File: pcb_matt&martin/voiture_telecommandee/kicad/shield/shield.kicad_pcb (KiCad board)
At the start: 2 copper layers, 100 x 100 mm, 13 parts, among them J2 Bluetooth, U1 COM-09032

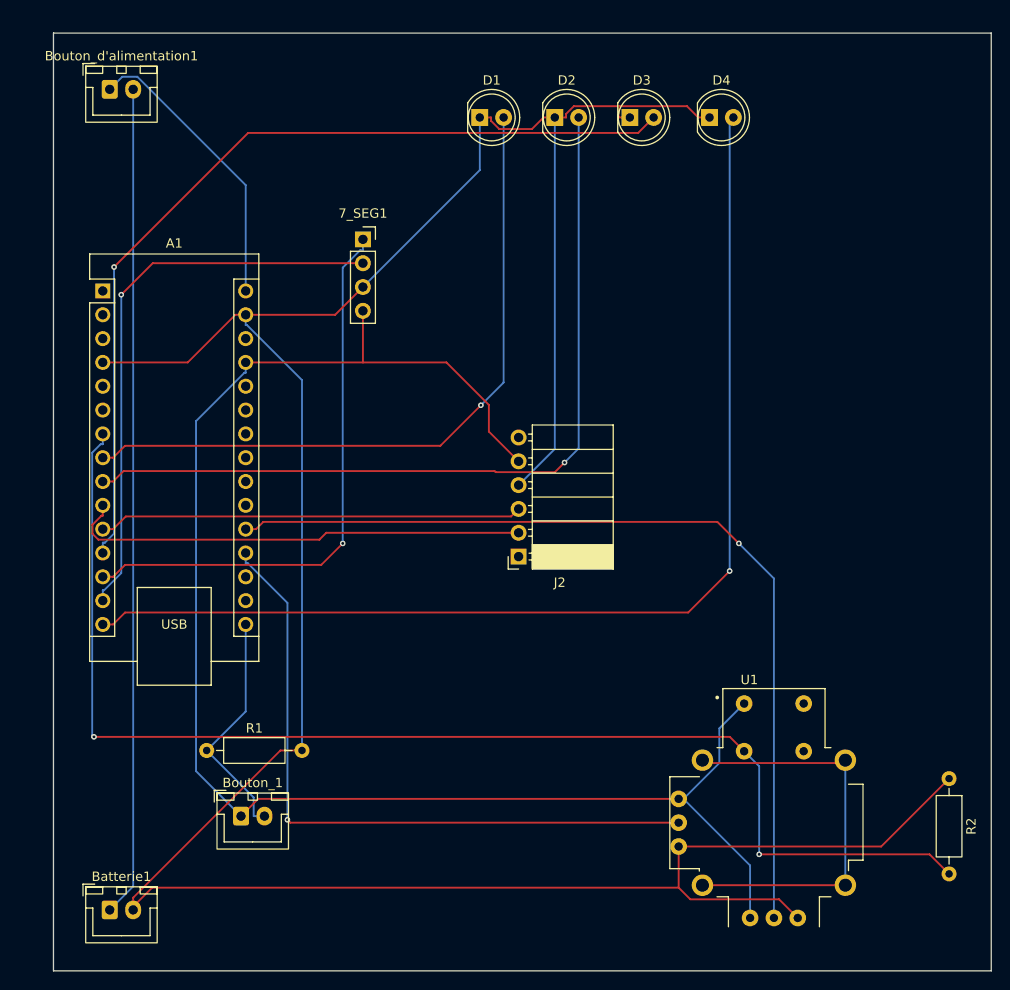
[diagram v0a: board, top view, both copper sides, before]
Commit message: bon euuuuu y'a bcp de changements
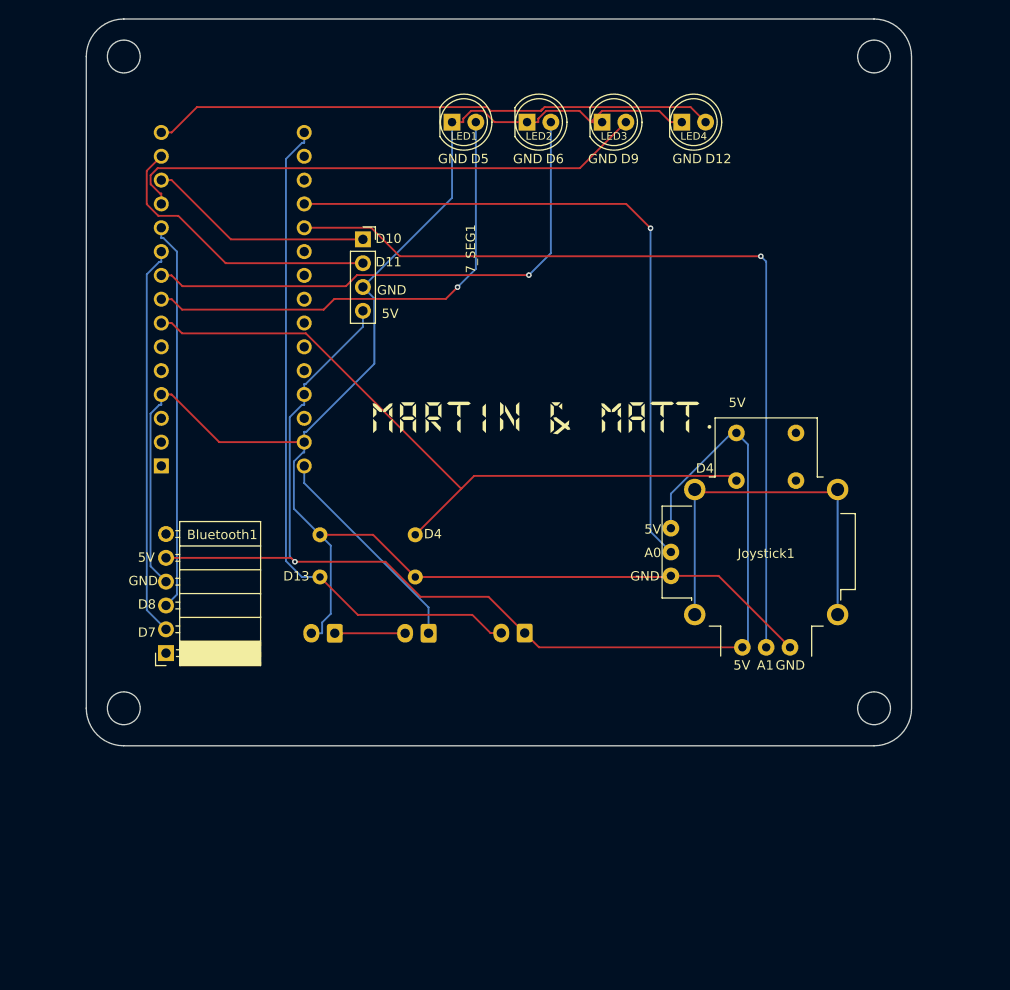
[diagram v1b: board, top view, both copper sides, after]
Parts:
- ARDUINO1: renamed from A1; moved to B.Cu
- Batterie1, R1, R2: moved to B.Cu
- Bouton1: renamed from Bouton_1; moved to B.Cu
- Btn_alim1: renamed from Bouton_d'alimentation1; moved to B.Cu
- moved R2 71.9 mm to (116.4, 104.0), turned to 0 degrees
- moved Btn_alim1 67.2 mm to (128.0, 114.5), turned to 180 degrees
- moved Bluetooth1 39.0 mm to (100.0, 116.6)
- moved Batterie1 38.0 mm to (118.0, 114.5), turned to 180 degrees
- moved Bouton1 36.0 mm to (138.2, 114.5), turned to 180 degrees
- moved Joystick1 28.9 mm to (164.0, 105.8)
- moved R1 22.1 mm to (116.4, 108.5)
- moved ARDUINO1 19.7 mm to (99.5, 96.7)
- moved LED1 3.00 mm to (130.5, 60.0)
- moved LED2 3.00 mm to (138.5, 60.0)
- moved LED3 3.00 mm to (146.5, 60.0)
- moved LED4 3.00 mm to (155.0, 60.0)
- renumbered J2 to Bluetooth1, U1 to Joystick1, D1 to LED1, D2 to LED2, D3 to LED3, D4 to LED4
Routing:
- net GND: track 308.6 -> 188.8 mm
- net /BTN_BATT_IN: track 88.5 -> 7.50 mm
- net /<NO NET>: track 136.5 -> 76.4 mm, vias 2 -> 0
- net /LED_4: track 117.7 -> 60.4 mm, vias 1 -> 0
- net /BTN_1: track 25.4 -> 72.8 mm
- net /LED_3: track 95.3 -> 56.6 mm, vias 1 -> 0
- net +5V: track 169.7 -> 132.8 mm, vias 0 -> 1
- net /7_SEG_CLK: track 60.5 -> 24.1 mm, vias 1 -> 0
- net /LED_2: track 87.9 -> 57.4 mm
- net /7_SEG_DIO: track 60.7 -> 31.4 mm, vias 1 -> 0
- net /LED_1: track 74.3 -> 51.4 mm
- net /BTN_BATT_OUT: track 31.1 -> 23.3 mm
- net /BTH_RX: track 49.6 -> 41.9 mm
- net /BTH_TX: track 45.2 -> 41.6 mm
- net /H2: track 95.3 -> 91.9 mm
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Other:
- board size 100 x 100 mm -> 88 x 77.5 mm
- board text added: "5V"
- board text added: "<->"
- board text added: "A0"
- board text added: "A1"
- board text added: "D10"
- board text added: "D11"
- board text added: "D12"
- board text added: "D13"
- board text added: "D4"
- board text added: "D5"
- board text added: "D6"
- board text added: "D7"
- board text added: "D8"
- board text added: "D9"
- board text added: "GND"
- board text added: "V.IN"
